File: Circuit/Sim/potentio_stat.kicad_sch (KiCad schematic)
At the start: 16 parts, among them U1 ${SIM.PARAMS}, U2 ${SIM.PARAMS}, U3 ${SIM.PARAMS}, U4 ${SIM.PARAMS}, U5 ${SIM.PARAMS}, U6 ${SIM.PARAMS}, U7 ${SIM.PARAMS}, U8 ${SIM.PARAMS}, U9 ${SIM.PARAMS}

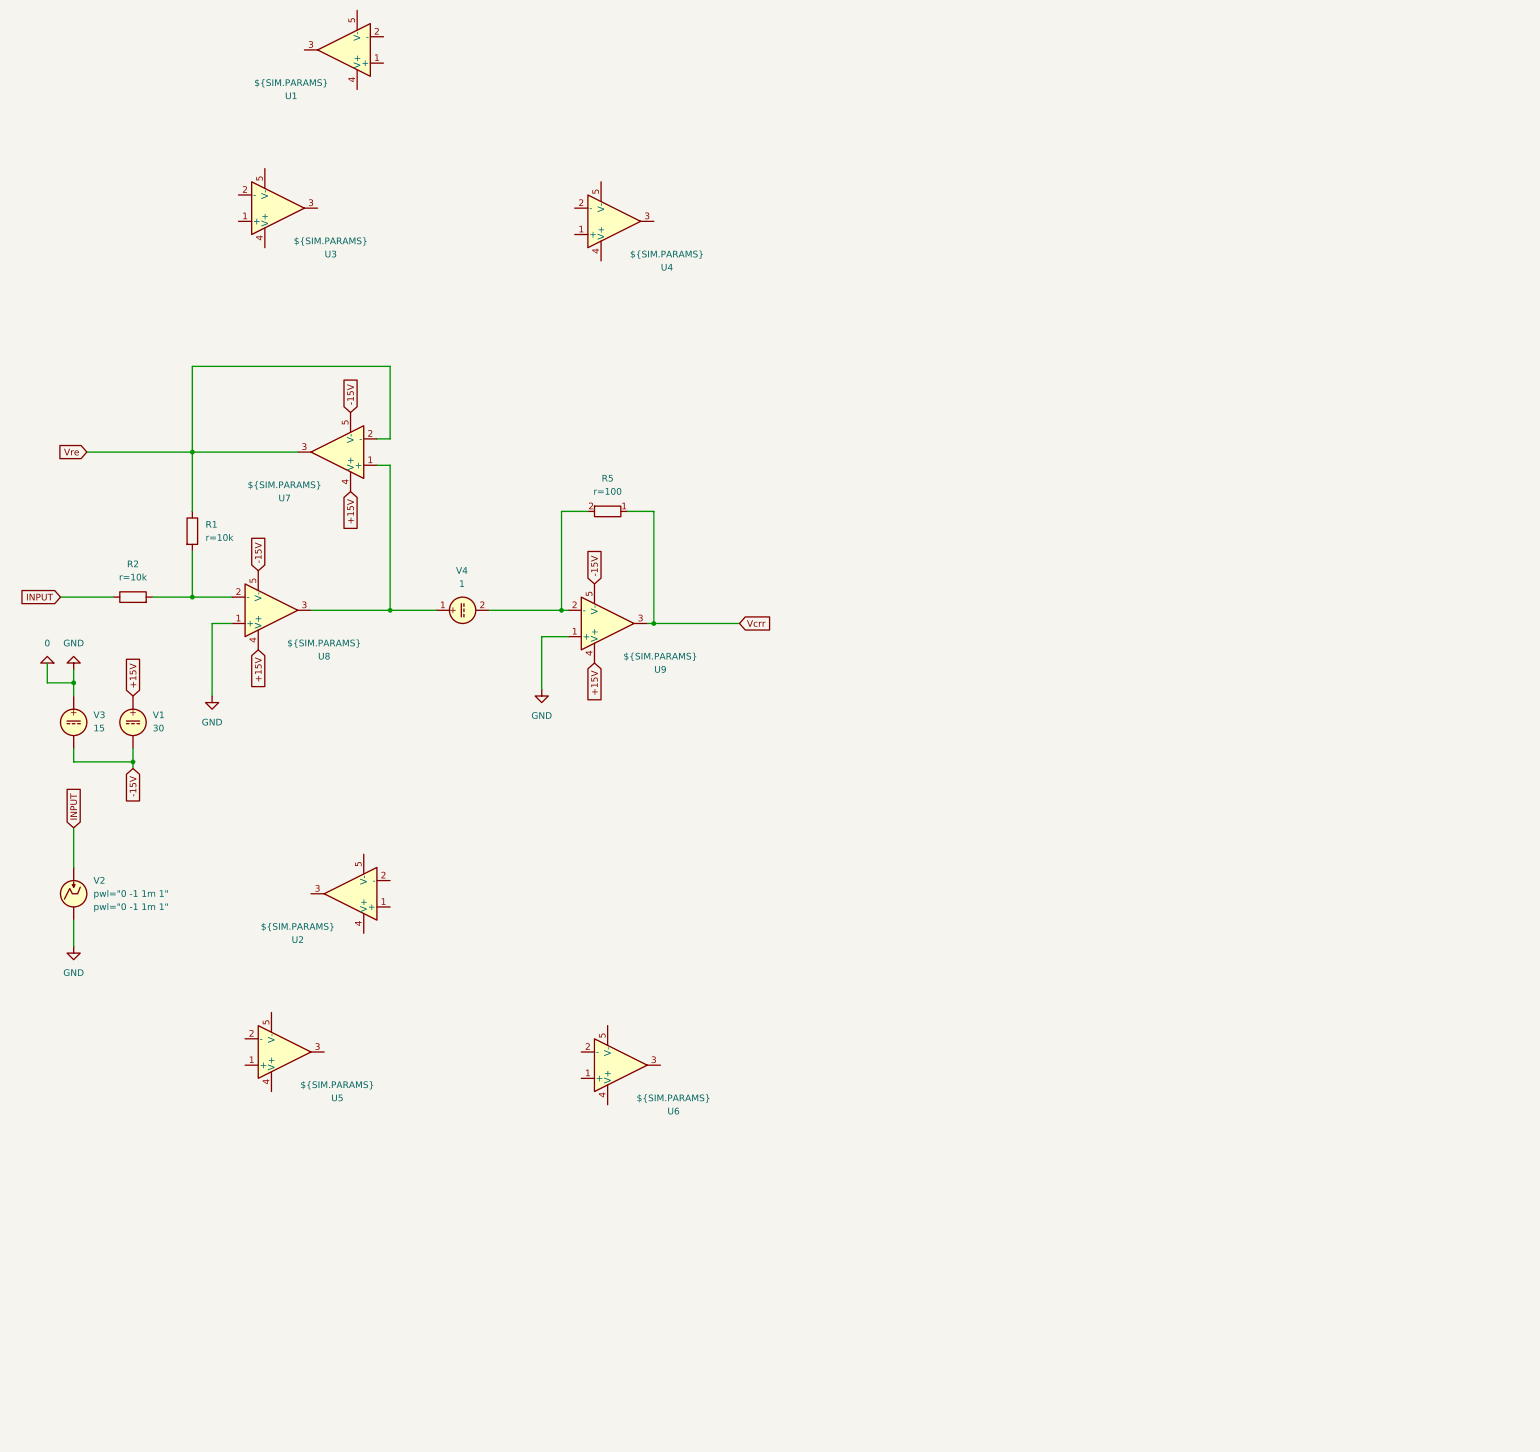
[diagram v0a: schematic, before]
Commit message: 電気化学インピーダンス用アップデート
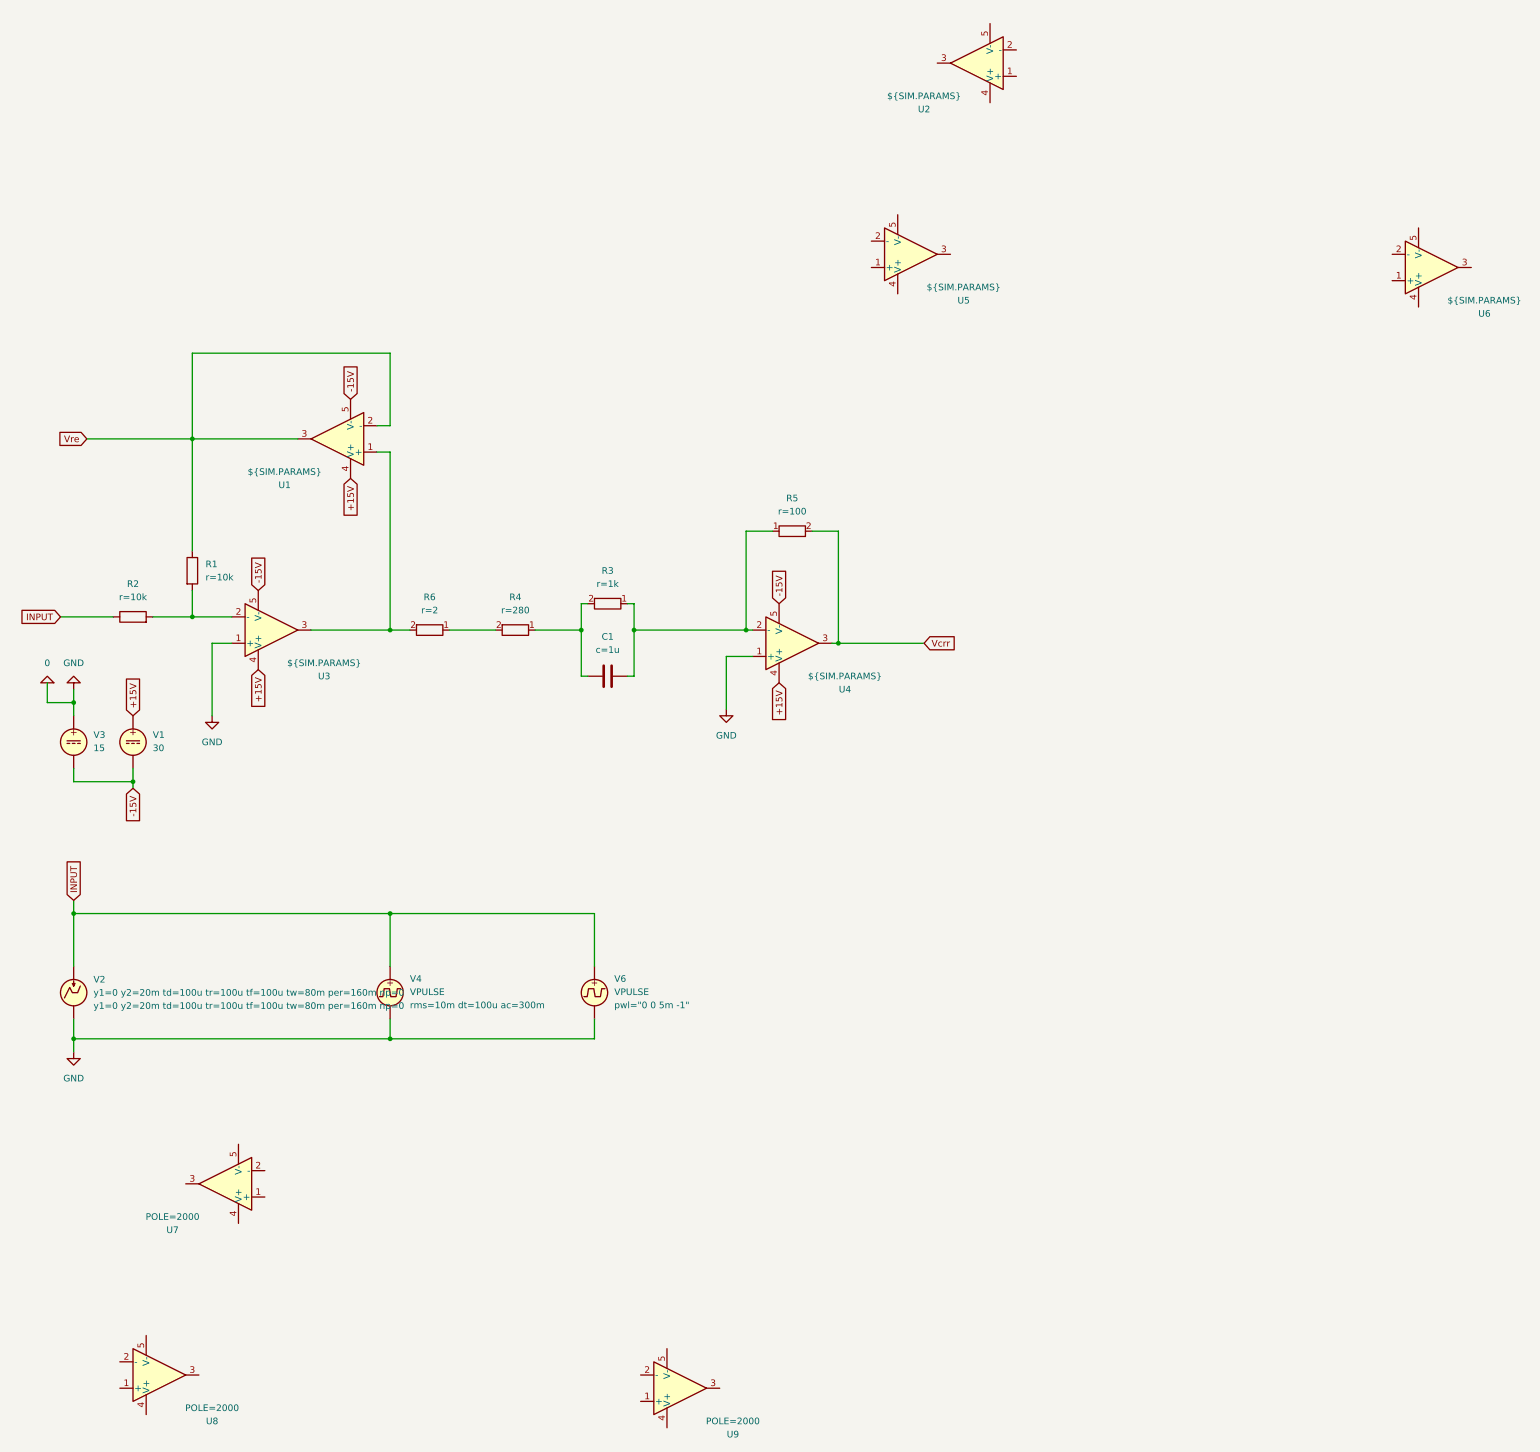
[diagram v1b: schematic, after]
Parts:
- removed V4: 1, symbol Simulation_SPICE:VDC
- added C1: ${SIM.PARAMS}, symbol Device:C
- added R3, R4, R6: ${SIM.PARAMS}, symbol Device:R
- added V4, V6: VPULSE, symbol Simulation_SPICE:VPULSE
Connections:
- net +15V: now also U1.4 (V+), U3.4 (V+), U4.4 (V+); no longer U7.4 (V+), U8.4 (V+), U9.4 (V+)
- net -15V: now also U1.5 (V-), U3.5 (V-), U4.5 (V-); no longer U7.5 (V-), U8.5 (V-), U9.5 (V-)
- net 0: now also U3.1 (+), U4.1 (+), V4.2, V6.2; no longer U8.1 (+), U9.1 (+)
- net INPUT: now also V4.1, V6.1
- net Vcrr: now also R5.2, U4.3; no longer R5.1, U9.3
- net Vre: now also U1.2 (-), U1.3; no longer U7.2 (-), U7.3
- net at U4.2 (-): now also R5.1, C1.2, R3.1
- net at U7.1 (+): no longer U8.3
- net at U9.2 (-): no longer R5.2
- net at R1.2, R2.2: now also U3.2 (-); no longer U8.2 (-)
- net at U3.3: now also U1.1 (+), R6.2
- new net: C1.1, R3.2, R4.1
- new net: R4.2, R6.1
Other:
- moved on the sheet: R1, R2, R5, U1, U3, U4, V1, V2, V3
